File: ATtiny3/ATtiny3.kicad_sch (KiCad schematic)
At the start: 8 parts, among them J1 LEDOUT1, J2 LEDOUT1, J3 POWER, U1 ATtiny824-X, U2 AP2127K-3.3

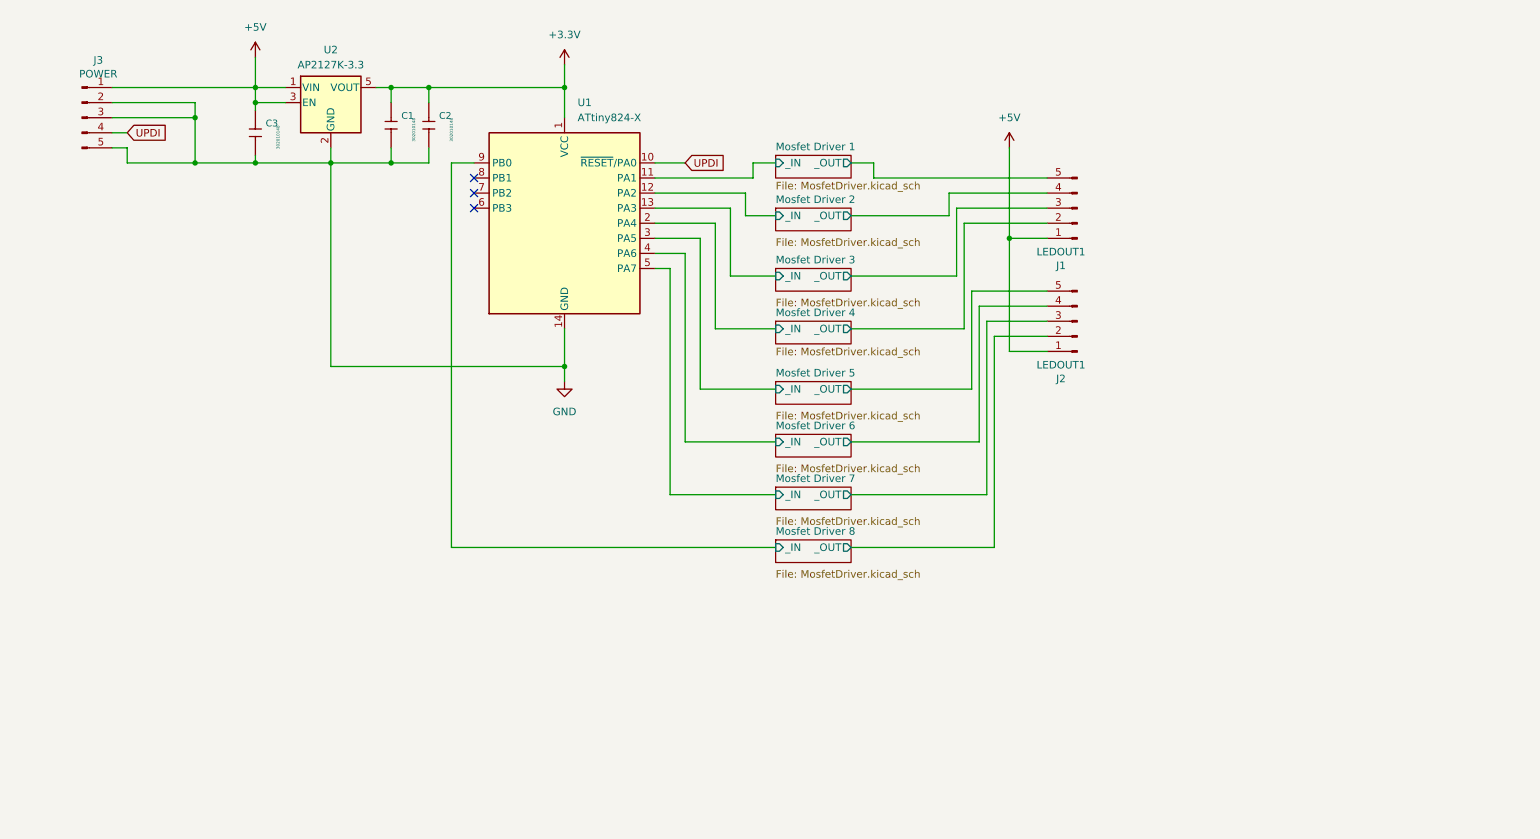
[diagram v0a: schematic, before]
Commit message: Primo ordine JLCPCB
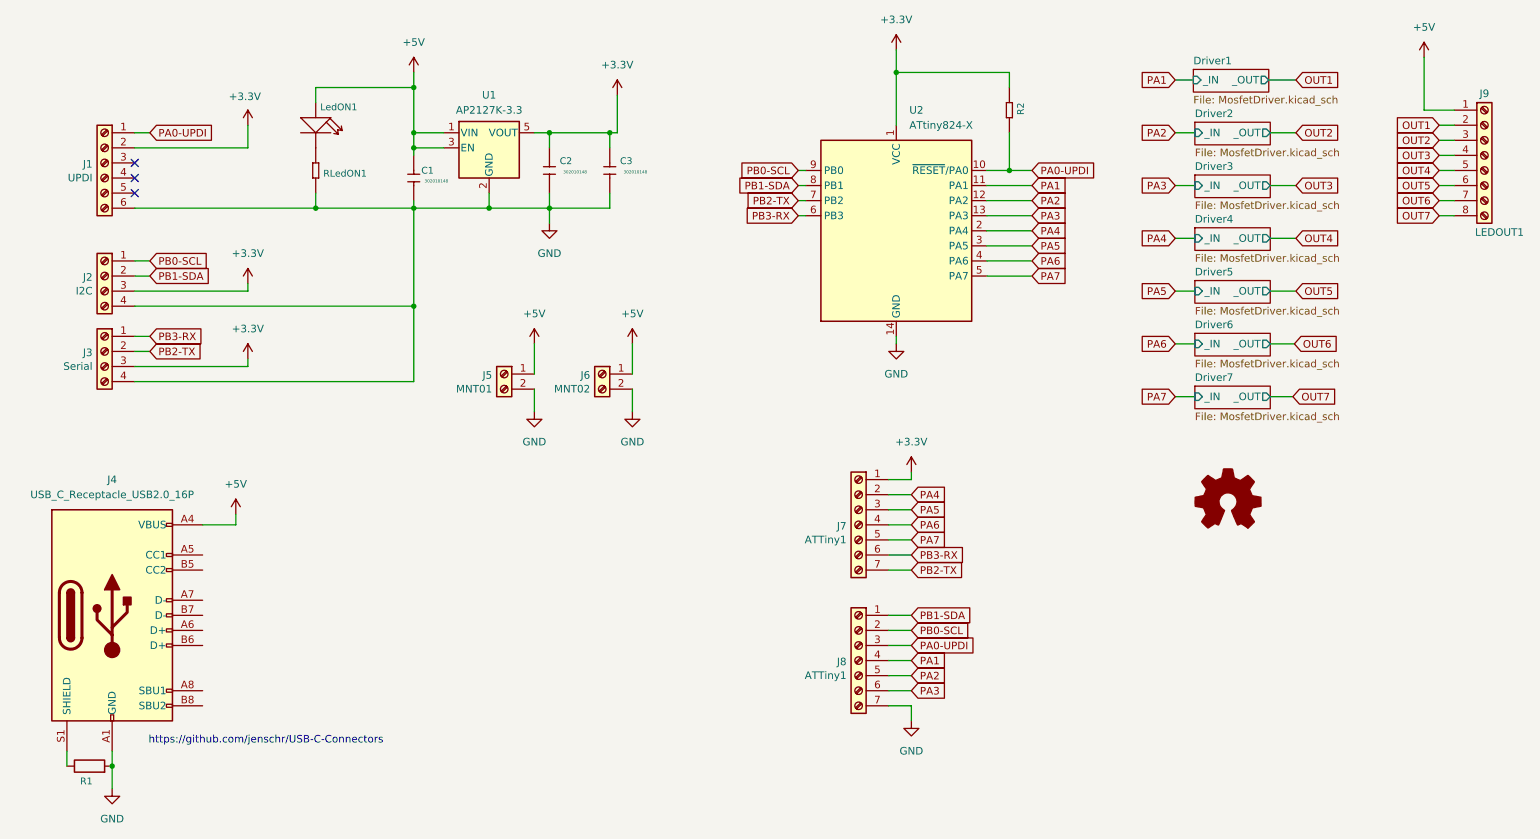
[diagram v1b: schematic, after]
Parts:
- removed J2: LEDOUT1, Connector_JST:JST_EH_B5B-EH-A_1x05_P2.50mm_Vertical, symbol ULN2803-Mosfet-S2-Mini-rescue:Conn_01x05_Male-Connector
- removed J3: POWER, Connector_JST:JST_EH_B5B-EH-A_1x05_P2.50mm_Vertical, symbol ULN2803-Mosfet-S2-Mini-rescue:Conn_01x05_Male-Connector
- added J1: UPDI, Connector_PinHeader_2.54mm:PinHeader_2x03_P2.54mm_Vertical, symbol Connector:Screw_Terminal_01x06
- added J2: I2C, Connector_PinHeader_2.54mm:PinHeader_1x04_P2.54mm_Vertical, symbol Connector:Screw_Terminal_01x04
- added J3: Serial, Connector_PinHeader_2.54mm:PinHeader_1x04_P2.54mm_Vertical, symbol Connector:Screw_Terminal_01x04
- added J4: USB_C_Receptacle_USB2.0_16P, Library-USB:TYPE-C-31-M-12, symbol Connector:USB_C_Receptacle_USB2.0_16P
- added J5: MNT01, Connector_PinHeader_2.54mm:PinHeader_1x02_P2.54mm_Vertical, symbol Connector:Screw_Terminal_01x02
- added J6: MNT02, Connector_PinHeader_2.54mm:PinHeader_1x02_P2.54mm_Vertical, symbol Connector:Screw_Terminal_01x02
- added J7, J8: ATTiny1, Connector_PinHeader_2.54mm:PinHeader_1x07_P2.54mm_Vertical, symbol Connector:Screw_Terminal_01x07
- added L1: Logo_Open_Hardware_Small, Symbol:OSHW-Logo_5.7x6mm_SilkScreen, symbol Graphic:Logo_Open_Hardware_Small
- added LedON1: SMD-LED-CLEAR-RED_0805_, LED_SMD:LED_0805_2012Metric, symbol ULN2803-Mosfet-S2-Mini-rescue:SMD-LED-CLEAR-RED_0805_-OPL_Opto
- added R1: 1M, Resistor_THT:R_Axial_DIN0204_L3.6mm_D1.6mm_P5.08mm_Horizontal, symbol Device:R
- added R2: 10K, Resistor_SMD:R_0805_2012Metric, symbol ULN2803-Mosfet-S2-Mini-rescue:SMD-RES-4.7K-5%-1_8W_0805_-OPL_Resistor
- added RLedON1: SMD-RES-220R-5%-1_8W_0805_, Resistor_SMD:R_0805_2012Metric, symbol ULN2803-Mosfet-S2-Mini-rescue:SMD-RES-220R-5%-1_8W_0805_-OPL_Resistor
- C1: renamed from C3; LCSC C126586 -> C15850
- C2: renamed from C1; LCSC C126586 -> C15850
- C3: renamed from C2; LCSC C126586 -> C15850
- J9: renamed from J1; footprint Connector_JST:JST_EH_B5B-EH-A_1x05_P2.50mm_Vertical -> Connector_PinHeader_2.54mm:PinHeader_1x08_P2.54mm_Vertical; symbol ULN2803-Mosfet-S2-Mini-rescue:Conn_01x05_Male-Connector -> Connector:Screw_Terminal_01x08; now left out of the parts list
- U1: renamed from U2; LCSC (none) -> C156285
- U2: renamed from U1; LCSC (none) -> C3237505; now left out of the parts list
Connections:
- net +3.3V: now also J1.2 (Pin_2), J2.3 (Pin_3), J3.3 (Pin_3), J7.1 (Pin_1), R2.1
- net +5V: now also J4.A4 (VBUS), J4.A9 (VBUS), J4.B4 (VBUS), J4.B9 (VBUS), J5.1 (Pin_1), J6.1 (Pin_1), LedON1.1 (+)
- net GND: now also J1.6 (Pin_6), J2.4 (Pin_4), J3.4 (Pin_4), J4.A1 (GND), J4.A12 (GND), J4.B1 (GND), J4.B12 (GND), J5.2 (Pin_2), J6.2 (Pin_2), J8.7 (Pin_7), R1.2, RLedON1.2
- net PB3-RX: now reaches U2.6 (PB3)
- net PB3-RX: now also J3.1 (Pin_1), J7.6 (Pin_6)
- net PB2-TX: now reaches U2.7 (PB2)
- net PB2-TX: now also J3.2 (Pin_2), J7.7 (Pin_7)
- net PB1-SDA: now reaches U2.8 (PB1)
- net PB1-SDA: now also J2.2 (Pin_2), J8.1 (Pin_1)
- net Mosfet Driver 1/_IN renamed PA1
- net PA1: now also J8.4 (Pin_4)
- net Mosfet Driver 1/_OUT renamed OUT4
- net Mosfet Driver 2/_IN renamed PA2
- net PA2: now also J8.5 (Pin_5)
- net Mosfet Driver 2/_OUT renamed OUT3
- net Mosfet Driver 3/_IN renamed PA3
- net PA3: now also J8.6 (Pin_6)
- net Mosfet Driver 3/_OUT renamed OUT2
- net Mosfet Driver 4/_IN renamed PA4
- net PA4: now also J7.2 (Pin_2)
- net Mosfet Driver 4/_OUT renamed OUT1
- net Mosfet Driver 5/_IN renamed PA5
- net PA5: now also J7.3 (Pin_3)
- net Mosfet Driver 6/_IN renamed PA6
- net PA6: now also J7.4 (Pin_4)
- net Mosfet Driver 7/_IN renamed PA7
- net PA7: now also J7.5 (Pin_5)
- net Mosfet Driver 8/_IN renamed PB0-SCL
- net PB0-SCL: now also J2.1 (Pin_1), J8.2 (Pin_2)
- net UPDI renamed PA0-UPDI
- net PA0-UPDI: now also J1.1 (Pin_1), J8.3 (Pin_3), R2.2
- new net: J4.S1 (SHIELD), R1.1
- new net: LedON1.2 (-), RLedON1.1
- new net OUT5: J9.6 (Pin_6)
- new net OUT6: J9.7 (Pin_7)
- new net OUT7: J9.8 (Pin_8)
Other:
- removed sheet Mosfet Driver 1
- removed sheet Mosfet Driver 2
- removed sheet Mosfet Driver 3
- removed sheet Mosfet Driver 4
- removed sheet Mosfet Driver 5
- removed sheet Mosfet Driver 6
- removed sheet Mosfet Driver 7
- removed sheet Mosfet Driver 8
- added sheet Driver1 (MosfetDriver.kicad_sch)
- added sheet Driver2 (MosfetDriver.kicad_sch)
- added sheet Driver3 (MosfetDriver.kicad_sch)
- added sheet Driver4 (MosfetDriver.kicad_sch)
- added sheet Driver5 (MosfetDriver.kicad_sch)
- added sheet Driver6 (MosfetDriver.kicad_sch)
- added sheet Driver7 (MosfetDriver.kicad_sch)
- note added: "https://github.com/jenschr/USB-C-Connectors"
- moved on the sheet: C1, C2, C3, U1, U2
